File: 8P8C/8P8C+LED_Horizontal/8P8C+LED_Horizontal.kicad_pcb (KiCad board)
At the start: 2 copper layers, 20.1 x 25.4 mm, 4 parts, among them J1 8P8C_LED_Shielded, J2 Conn_01x06, J3 Conn_01x06

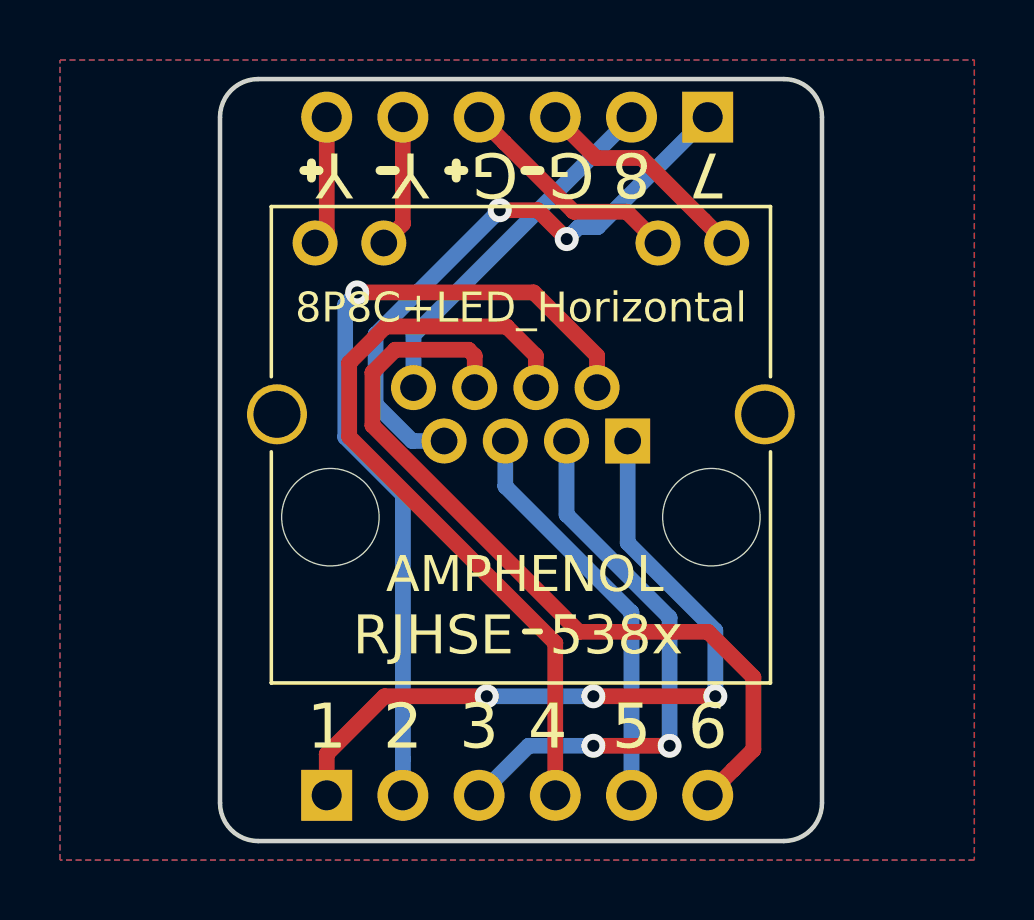
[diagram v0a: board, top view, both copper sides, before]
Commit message: Re-align pins
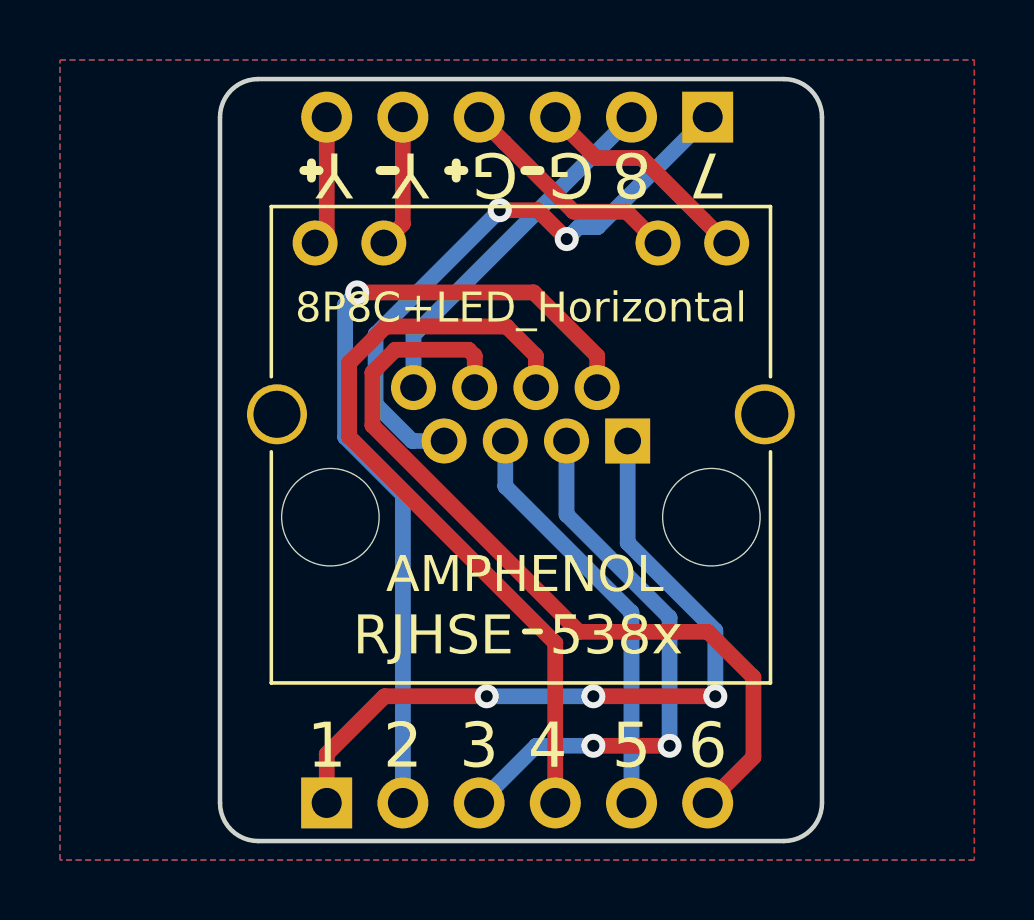
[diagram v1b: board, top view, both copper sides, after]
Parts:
- moved J2 0.25 mm to (134.6, 116.8)
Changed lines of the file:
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@@
     (thickness 1.6)
     (drawings 38)
-    (tracks 75)
+    (tracks 73)
     (zones 0)
     (modules 4)
@@
     (32 B.Adhes user)
     (33 F.Adhes user)
-    (34 B.Paste user)
+    (34 B.Paste user hide)
     (35 F.Paste user)
-    (36 B.SilkS user)
+    (36 B.SilkS user hide)
     (37 F.SilkS user)
     (38 B.Mask user)
@@
   )
   (module 8P8C+LED_Horizontal:PinHeader_1x06_P2.54mm_Vertical (layer B.Cu)
-    (at 134.62 116.586 270)
+    (at 134.62 116.84 270)
     (descr "Through hole straight pin header, 1x06, 2.54mm pitch, single row")
     (tags "Through hole pin header THT 1x06 2.54mm single row")
@@
     (effects (font (size 1.5 1.5) (thickness 0.3)))
   )
-  (gr_text 6 (at 147.32 114.3) (layer F.SilkS)
-    (effects (font (size 1.5 1.5) (thickness 0.3)))
-  )
-  (gr_text 5 (at 144.78 114.3) (layer F.SilkS)
-    (effects (font (size 1.5 1.5) (thickness 0.3)))
-  )
-  (gr_text 4 (at 141.986 114.3) (layer F.SilkS)
-    (effects (font (size 1.5 1.5) (thickness 0.3)))
-  )
-  (gr_text 3 (at 139.7 114.3) (layer F.SilkS)
-    (effects (font (size 1.5 1.5) (thickness 0.3)))
-  )
-  (gr_text 2 (at 137.16 114.3) (layer F.SilkS)
-    (effects (font (size 1.5 1.5) (thickness 0.3)))
-  )
-  (gr_text 1 (at 134.62 114.3) (layer F.SilkS)
+  (gr_text 6 (at 147.32 114.935) (layer F.SilkS)
+    (effects (font (size 1.5 1.5) (thickness 0.3)))
+  )
+  (gr_text 5 (at 144.78 114.935) (layer F.SilkS)
+    (effects (font (size 1.5 1.5) (thickness 0.3)))
+  )
+  (gr_text 4 (at 141.986 114.935) (layer F.SilkS)
+    (effects (font (size 1.5 1.5) (thickness 0.3)))
+  )
+  (gr_text 3 (at 139.7 114.935) (layer F.SilkS)
+    (effects (font (size 1.5 1.5) (thickness 0.3)))
+  )
+  (gr_text 2 (at 137.16 114.935) (layer F.SilkS)
+    (effects (font (size 1.5 1.5) (thickness 0.3)))
+  )
+  (gr_text 1 (at 134.62 114.935) (layer F.SilkS)
     (effects (font (size 1.5 1.5) (thickness 0.3)))
   )
@@
   (gr_arc (start 132.334 93.98) (end 132.334 92.71) (angle -90) (layer Edge.Cuts) (width 0.15))
   (gr_arc (start 149.86 93.98) (end 151.13 93.98) (angle -90) (layer Edge.Cuts) (width 0.15))
-  (segment (start 148.169999 115.736001) (end 147.32 116.586) (width 0.525) (layer F.Cu) (net 2))
+  (segment (start 148.844 115.316) (end 147.32 116.84) (width 0.525) (layer F.Cu) (net 2))
   (segment (start 147.33301 111.13801) (end 148.844 112.649) (width 0.525) (layer F.Cu) (net 2))
   (segment (start 143.01501 111.13801) (end 147.33301 111.13801) (width 0.525) (layer F.Cu) (net 2))
-  (segment (start 143.01501 111.125512) (end 143.01501 111.13801) (width 0.525) (layer F.Cu) (net 2))
-  (segment (start 148.844 112.649) (end 148.844 115.062) (width 0.525) (layer F.Cu) (net 2))
   (segment (start 139.553 101.93434) (end 139.351159 101.732499) (width 0.525) (layer F.Cu) (net 2))
+  (segment (start 148.844 112.649) (end 148.844 115.316) (width 0.525) (layer F.Cu) (net 2))
   (segment (start 139.553 102.995) (end 139.553 101.93434) (width 0.525) (layer F.Cu) (net 2))
   (segment (start 139.351159 101.732499) (end 136.906999 101.732499) (width 0.525) (layer F.Cu) (net 2))
+  (segment (start 143.01501 111.125512) (end 143.01501 111.13801) (width 0.525) (layer F.Cu) (net 2))
+  (segment (start 136.144 102.495498) (end 136.144 104.254502) (width 0.525) (layer F.Cu) (net 2))
   (segment (start 136.906999 101.732499) (end 136.144 102.495498) (width 0.525) (layer F.Cu) (net 2))
-  (segment (start 148.844 115.062) (end 148.169999 115.736001) (width 0.525) (layer F.Cu) (net 2))
-  (segment (start 136.144 102.495498) (end 136.144 104.254502) (width 0.525) (layer F.Cu) (net 2))
   (segment (start 136.144 104.254502) (end 143.01501 111.125512) (width 0.525) (layer F.Cu) (net 2))
   (segment (start 135.36899 102.174479) (end 135.36899 104.63499) (width 0.525) (layer F.Cu) (net 3))
@@
   (segment (start 143.633 102.995) (end 143.633 101.93434) (width 0.525) (layer F.Cu) (net 4))
   (segment (start 143.633 101.93434) (end 141.52066 99.822) (width 0.525) (layer F.Cu) (net 4))
-  (segment (start 137.16 115.383919) (end 137.16 116.586) (width 0.525) (layer B.Cu) (net 4))
-  (segment (start 137.16 106.568498) (end 137.16 115.383919) (width 0.525) (layer B.Cu) (net 4))
   (segment (start 135.236001 104.644499) (end 137.16 106.568498) (width 0.525) (layer B.Cu) (net 4))
   (segment (start 135.236001 100.221999) (end 135.236001 104.644499) (width 0.525) (layer B.Cu) (net 4))
   (segment (start 135.636 99.822) (end 135.236001 100.221999) (width 0.525) (layer B.Cu) (net 4))
+  (segment (start 137.16 106.568498) (end 137.16 116.84) (width 0.525) (layer B.Cu) (net 4))
   (via (at 140.388265 97.081265) (size 0.8) (drill 0.4) (layers F.Cu B.Cu) (net 5))
   (segment (start 136.250499 101.219031) (end 140.388265 97.081265) (width 0.525) (layer B.Cu) (net 5))
@@
   (via (at 143.51 114.935) (size 0.8) (drill 0.4) (layers F.Cu B.Cu) (net 7))
   (segment (start 146.05 114.935) (end 143.51 114.935) (width 0.525) (layer F.Cu) (net 7))
-  (segment (start 141.351 114.935) (end 139.7 116.586) (width 0.525) (layer B.Cu) (net 7))
-  (segment (start 143.51 114.935) (end 141.351 114.935) (width 0.525) (layer B.Cu) (net 7))
+  (segment (start 141.605 114.935) (end 139.7 116.84) (width 0.525) (layer B.Cu) (net 7))
+  (segment (start 143.51 114.935) (end 141.605 114.935) (width 0.525) (layer B.Cu) (net 7))
   (via (at 147.574 113.284) (size 0.8) (drill 0.4) (layers F.Cu B.Cu) (net 8))
   (segment (start 147.574 111.091948) (end 147.574 113.284) (width 0.525) (layer B.Cu) (net 8))
